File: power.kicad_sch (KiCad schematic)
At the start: 38 parts, among them IC3 LP5912-3.3DRVR, U2 BQ24075RGT, U3 LP5907SNX-3.3/NOPB, U4 LP5907SNX-3.3/NOPB, U5 LP5907SNX-1.8/NOPB, U6 LP5907SNX-3.3/NOPB, U7 LP5907SNX-1.8/NOPB

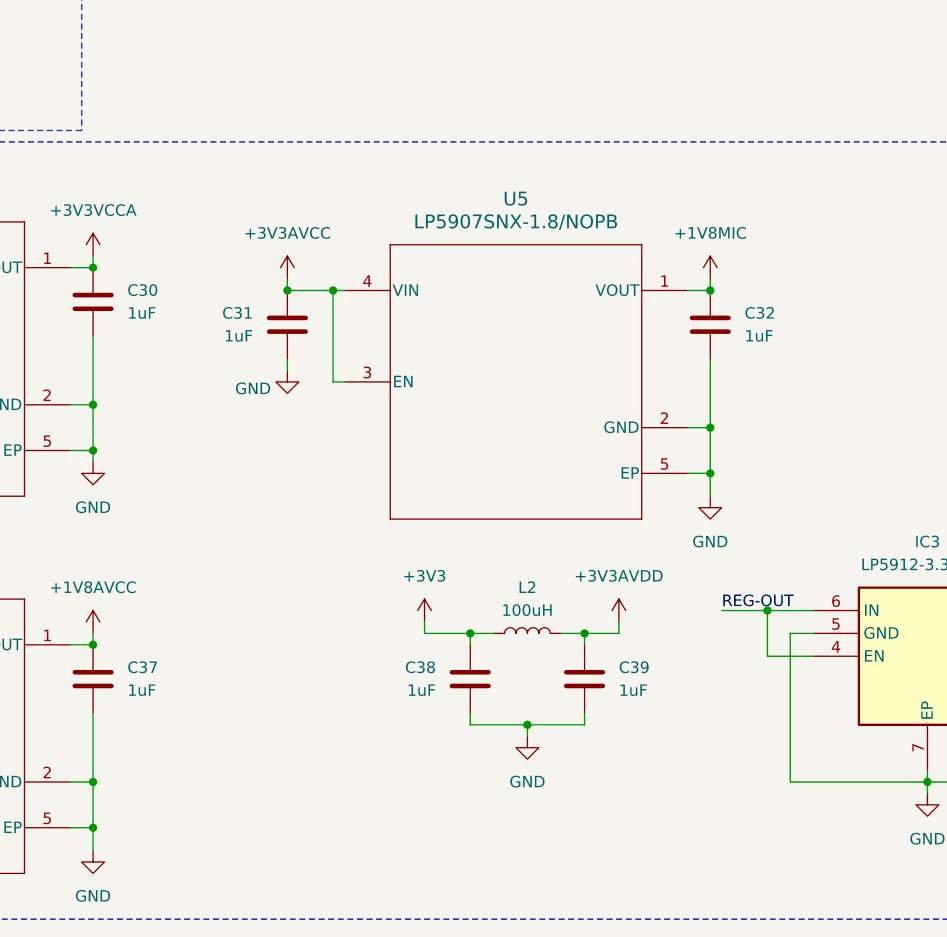
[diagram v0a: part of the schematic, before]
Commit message: small fixes
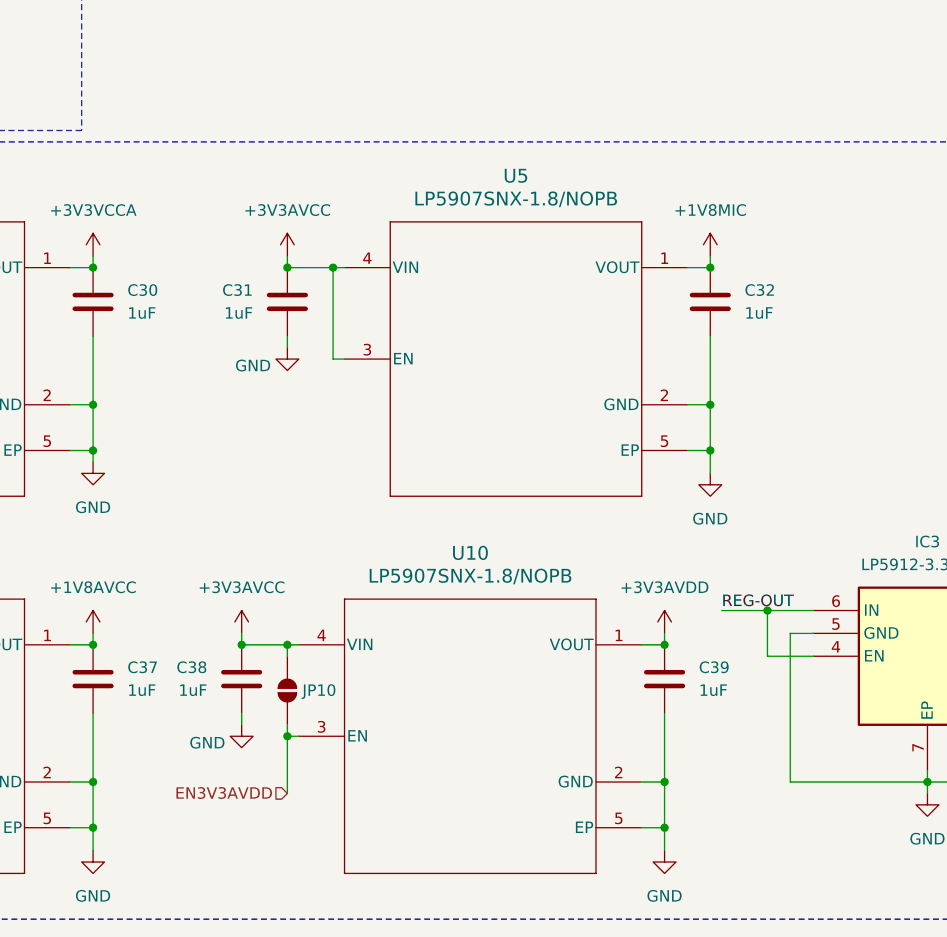
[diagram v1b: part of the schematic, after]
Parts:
- removed L2: 100uH, Inductor_SMD:L_TDK_MLZ2012_h1.25mm, symbol Device:L
- added JP10: SolderJumper_2_Open, Jumper:SolderJumper-2_P1.3mm_Open_RoundedPad1.0x1.5mm, symbol Jumper:SolderJumper_2_Open
- added U10: LP5907SNX-1.8/NOPB, Package_SON:Texas_X2SON-4_1x1mm_P0.65mm, symbol LP5907SNX-1-8-NOPB:LP5907SNX-1.8_NOPB
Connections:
- net +3V3: no longer C38.1
- net +3V3AVCC: now also C38.1, JP10.1 (A), U10.4 (VIN)
- net +3V3AVDD: now also U10.1 (VOUT)
- net GND: now also U10.2 (GND), U10.5 (EP)
- new net EN3V3AVDD: JP10.2 (B), U10.3 (EN)
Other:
- moved on the sheet: C31, C32, U5
